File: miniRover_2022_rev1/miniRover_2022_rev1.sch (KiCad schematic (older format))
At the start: 5 parts, among them J1 XT60-M, U1 OKI

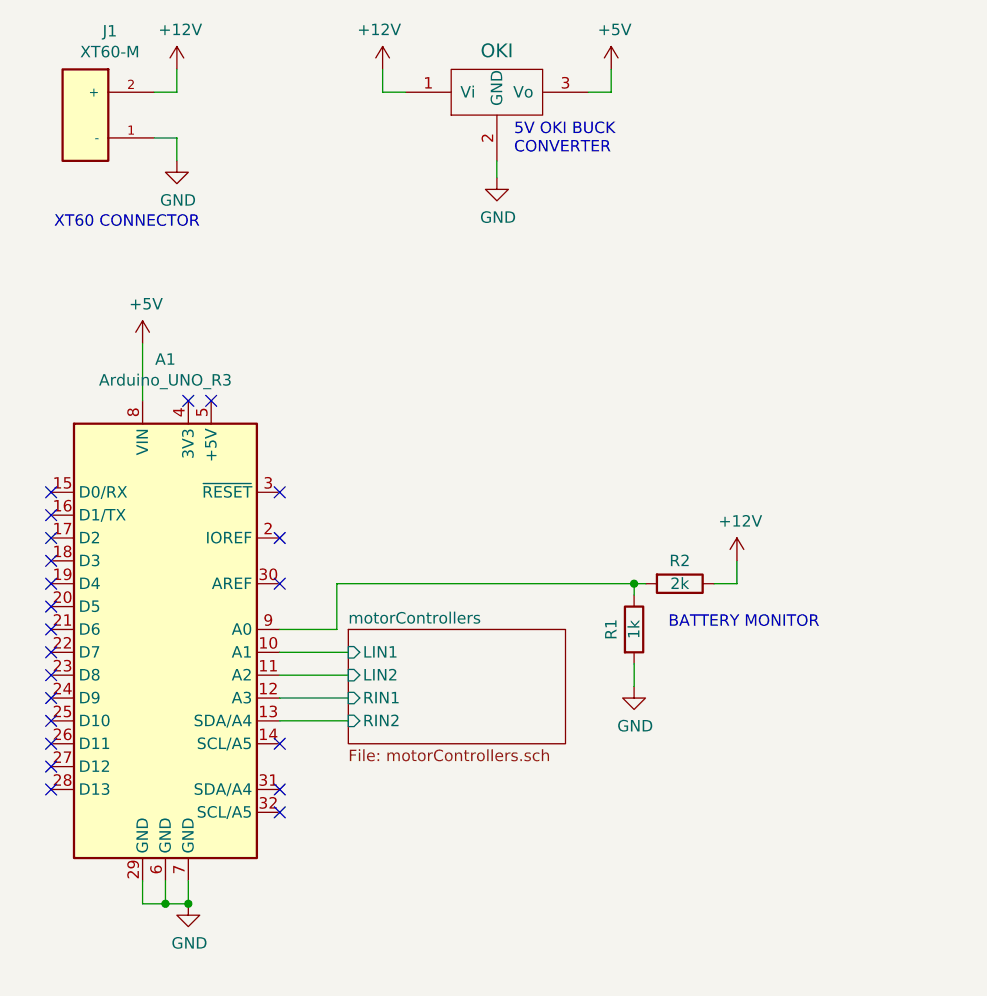
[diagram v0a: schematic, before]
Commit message: rev1 finished, will be reviewing over the following days
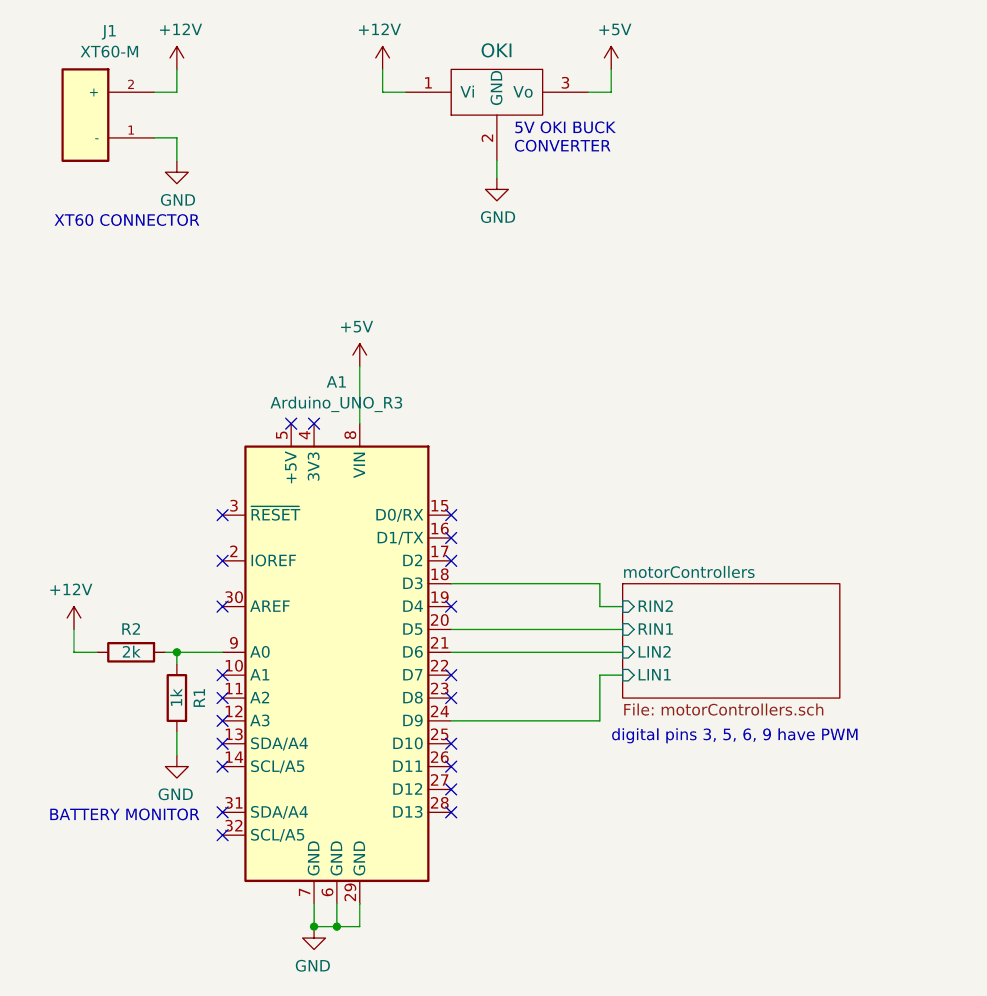
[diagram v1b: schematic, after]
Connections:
- net motorControllers/LIN1: now also A1.24 (D9); no longer A1.10 (A1)
- net motorControllers/LIN2: now also A1.21 (D6); no longer A1.11 (A2)
- net motorControllers/RIN1: now also A1.20 (D5); no longer A1.12 (A3)
- net motorControllers/RIN2: now also A1.18 (D3); no longer A1.13 (SDA/A4)
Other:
- note added: "digital pins 3, 5, 6, 9 have PWM"
- moved on the sheet: A1, R1, R2
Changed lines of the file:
@@
 Wire Wire Line
 	1100 1000 1100 1100
-$Comp
-L MCU_Module:Arduino_UNO_R3 A1
-U 1 1 60EDF96D
-P 1050 3150
-F 0 "A1" H 1050 4331 50  0000 C CNN
-F 1 "Arduino_UNO_R3" H 1050 4240 50  0000 C CNN
-F 2 "Module:Arduino_UNO_R3_WithMountingHoles" H 1050 3150 50  0001 C CIN
-F 3 "https://www.arduino.cc/en/Main/arduinoBoardUno" H 1050 3150 50  0001 C CNN
-	1    1050 3150
-	1    0    0    -1
-$EndComp
-Wire Wire Line
-	1550 3250 1850 3250
-Wire Wire Line
-	1550 3350 1850 3350
-Wire Wire Line
-	1550 3450 1850 3450
-Wire Wire Line
-	1550 3550 1850 3550
-NoConn ~ 1550 2550
-NoConn ~ 1550 2750
-NoConn ~ 1550 2950
-NoConn ~ 1550 3850
-NoConn ~ 1550 3950
+NoConn ~ 1300 2650
+NoConn ~ 1300 2850
+NoConn ~ 1300 3050
+NoConn ~ 1300 3950
+NoConn ~ 1300 4050
 $Comp
 L power:GND #PWR0106
 U 1 1 60F80F90
-P 1150 4350
-F 0 "#PWR0106" H 1150 4100 50  0001 C CNN
-F 1 "GND" H 1155 4177 50  0000 C CNN
-F 2 "" H 1150 4350 50  0001 C CNN
-F 3 "" H 1150 4350 50  0001 C CNN
-	1    1150 4350
-	1    0    0    -1
-$EndComp
-Wire Wire Line
-	950  4250 950  4350
-Wire Wire Line
-	950  4350 1050 4350
-Wire Wire Line
-	1150 4250 1150 4350
-Connection ~ 1150 4350
-Wire Wire Line
-	1050 4250 1050 4350
-Connection ~ 1050 4350
-Wire Wire Line
-	1050 4350 1150 4350
-Wire Wire Line
-	950  1900 950  2150
+P 1700 4450
+F 0 "#PWR0106" H 1700 4200 50  0001 C CNN
+F 1 "GND" H 1705 4277 50  0000 C CNN
+F 2 "" H 1700 4450 50  0001 C CNN
+F 3 "" H 1700 4450 50  0001 C CNN
+	1    1700 4450
+	-1   0    0    -1
+$EndComp
+Wire Wire Line
+	1900 4350 1900 4450
+Wire Wire Line
+	1900 4450 1800 4450
+Wire Wire Line
+	1700 4350 1700 4450
+Connection ~ 1700 4450
+Wire Wire Line
+	1800 4350 1800 4450
+Connection ~ 1800 4450
+Wire Wire Line
+	1800 4450 1700 4450
+Wire Wire Line
+	1900 2000 1900 2250
 $Comp
 L power:+5V #PWR0107
 U 1 1 60F82284
-P 950 1900
-F 0 "#PWR0107" H 950 1750 50  0001 C CNN
-F 1 "+5V" H 965 2073 50  0000 C CNN
-F 2 "" H 950 1900 50  0001 C CNN
-F 3 "" H 950 1900 50  0001 C CNN
-	1    950  1900
-	1    0    0    -1
-$EndComp
-Wire Wire Line
-	1550 3150 1800 3150
-Wire Wire Line
-	1800 3150 1800 2950
-Wire Wire Line
-	1800 2950 3100 2950
+P 1900 2000
+F 0 "#PWR0107" H 1900 1850 50  0001 C CNN
+F 1 "+5V" H 1915 2173 50  0000 C CNN
+F 2 "" H 1900 2000 50  0001 C CNN
+F 3 "" H 1900 2000 50  0001 C CNN
+	1    1900 2000
+	-1   0    0    -1
+$EndComp
 $Comp
 L Device:R R2
 U 1 1 60F82ECB
-P 3300 2950
-F 0 "R2" V 3200 2950 50  0000 C CNN
-F 1 "2k" V 3300 2950 50  0000 C CNN
-F 2 "Resistor_SMD:R_0603_1608Metric_Pad1.05x0.95mm_HandSolder" V 3230 2950 50  0001 C CNN
-F 3 "~" H 3300 2950 50  0001 C CNN
-	1    3300 2950
-	0    1    1    0
+P 900 3250
+F 0 "R2" V 800 3250 50  0000 C CNN
+F 1 "2k" V 900 3250 50  0000 C CNN
+F 2 "Resistor_SMD:R_0603_1608Metric_Pad1.05x0.95mm_HandSolder" V 830 3250 50  0001 C CNN
+F 3 "~" H 900 3250 50  0001 C CNN
+	1    900  3250
+	0    -1   1    0
 $EndComp
 $Comp
 L Device:R R1
 U 1 1 60F837E9
-P 3100 3150
-F 0 "R1" V 3000 3150 50  0000 C CNN
-F 1 "1k" V 3100 3150 50  0000 C CNN
-F 2 "Resistor_SMD:R_0603_1608Metric_Pad1.05x0.95mm_HandSolder" V 3030 3150 50  0001 C CNN
-F 3 "~" H 3100 3150 50  0001 C CNN
-	1    3100 3150
-	1    0    0    -1
-$EndComp
-Wire Wire Line
-	3100 3000 3100 2950
-Wire Wire Line
-	3150 2950 3100 2950
-Connection ~ 3100 2950
+P 1100 3450
+F 0 "R1" V 1000 3450 50  0000 C CNN
+F 1 "1k" V 1100 3450 50  0000 C CNN
+F 2 "Resistor_SMD:R_0603_1608Metric_Pad1.05x0.95mm_HandSolder" V 1030 3450 50  0001 C CNN
+F 3 "~" H 1100 3450 50  0001 C CNN
+	1    1100 3450
+	-1   0    0    -1
+$EndComp
+Wire Wire Line
+	1100 3300 1100 3250
+Wire Wire Line
+	1050 3250 1100 3250
 $Comp
 L power:GND #PWR0108
 U 1 1 60F84498
-P 3100 3400
-F 0 "#PWR0108" H 3100 3150 50  0001 C CNN
-F 1 "GND" H 3105 3227 50  0000 C CNN
-F 2 "" H 3100 3400 50  0001 C CNN
-F 3 "" H 3100 3400 50  0001 C CNN
-	1    3100 3400
-	1    0    0    -1
-$EndComp
-Wire Wire Line
-	3100 3300 3100 3400
-Wire Wire Line
-	3450 2950 3550 2950
-Wire Wire Line
-	3550 2950 3550 2850
+P 1100 3700
+F 0 "#PWR0108" H 1100 3450 50  0001 C CNN
+F 1 "GND" H 1105 3527 50  0000 C CNN
+F 2 "" H 1100 3700 50  0001 C CNN
+F 3 "" H 1100 3700 50  0001 C CNN
+	1    1100 3700
+	-1   0    0    -1
+$EndComp
+Wire Wire Line
+	1100 3600 1100 3700
+Wire Wire Line
+	750  3250 650  3250
+Wire Wire Line
+	650  3250 650  3150
 $Comp
 L power:+12V #PWR0109
 U 1 1 60F84D22
-P 3550 2850
-F 0 "#PWR0109" H 3550 2700 50  0001 C CNN
-F 1 "+12V" H 3565 3023 50  0000 C CNN
-F 2 "" H 3550 2850 50  0001 C CNN
-F 3 "" H 3550 2850 50  0001 C CNN
-	1    3550 2850
-	1    0    0    -1
-$EndComp
-NoConn ~ 550  3850
-NoConn ~ 550  3750
-NoConn ~ 550  3650
-NoConn ~ 550  3550
-NoConn ~ 550  3450
-NoConn ~ 550  3350
-NoConn ~ 550  3250
-NoConn ~ 550  3150
-NoConn ~ 550  3050
-NoConn ~ 550  2950
-NoConn ~ 550  2850
-NoConn ~ 550  2750
-NoConn ~ 550  2650
-NoConn ~ 550  2550
-NoConn ~ 1550 3650
+P 650 3150
+F 0 "#PWR0109" H 650 3000 50  0001 C CNN
+F 1 "+12V" H 665 3323 50  0000 C CNN
+F 2 "" H 650 3150 50  0001 C CNN
+F 3 "" H 650 3150 50  0001 C CNN
+	1    650  3150
+	-1   0    0    -1
+$EndComp
+NoConn ~ 2300 3950
+NoConn ~ 2300 3850
+NoConn ~ 2300 3750
+NoConn ~ 2300 3650
+NoConn ~ 2300 3450
+NoConn ~ 2300 3350
+NoConn ~ 2300 3050
+NoConn ~ 2300 2850
+NoConn ~ 2300 2750
+NoConn ~ 2300 2650
+NoConn ~ 1300 3750
 Text Notes 1200 1400 2    50   ~ 0
 XT60 CONNECTOR\n
@@
 Text Notes 2575 1075 0    50   ~ 0
 5V OKI BUCK\nCONVERTER
-Text Notes 3250 3150 0    50   ~ 0
+Text Notes 1200 4000 2    50   ~ 0
 BATTERY MONITOR
 $Sheet
-S 1850 3150 950  500
+S 3050 2950 950  500
 U 60F3E927
 F0 "motorControllers" 50
 F1 "motorControllers.sch" 50
-F2 "LIN1" I L 1850 3250 50
-F3 "LIN2" I L 1850 3350 50
-F4 "RIN1" I L 1850 3450 50
-F5 "RIN2" I L 1850 3550 50
+F2 "LIN1" I L 3050 3350 50
+F3 "LIN2" I L 3050 3250 50
+F4 "RIN1" I L 3050 3150 50
+F5 "RIN2" I L 3050 3050 50
 $EndSheet
-NoConn ~ 1150 2150
-NoConn ~ 1250 2150
+NoConn ~ 1700 2250
+NoConn ~ 1600 2250
+$Comp
+L MCU_Module:Arduino_UNO_R3 A1
+U 1 1 60EDF96D
+P 1800 3250
+F 0 "A1" H 1800 4431 50  0000 C CNN
+F 1 "Arduino_UNO_R3" H 1800 4340 50  0000 C CNN
+F 2 "Module:Arduino_UNO_R3_WithMountingHoles" H 1800 3250 50  0001 C CIN
+F 3 "https://www.arduino.cc/en/Main/arduinoBoardUno" H 1800 3250 50  0001 C CNN
+	1    1800 3250
+	-1   0    0    -1
+$EndComp
+Wire Wire Line
+	1300 3250 1100 3250
+Connection ~ 1100 3250
+NoConn ~ 1300 3350
+NoConn ~ 1300 3450
+NoConn ~ 1300 3550
+NoConn ~ 1300 3650
+Text Notes 3000 3650 0    50   ~ 0
+digital pins 3, 5, 6, 9 have PWM
+Wire Wire Line
+	3050 3250 2300 3250
+Wire Wire Line
+	2300 3150 3050 3150
+Wire Wire Line
+	3050 3050 2950 3050
+Wire Wire Line
+	2950 3050 2950 2950
+Wire Wire Line
+	2950 2950 2300 2950
+Wire Wire Line
+	2300 3550 2950 3550
+Wire Wire Line
+	2950 3550 2950 3350
+Wire Wire Line
+	2950 3350 3050 3350
 $EndSCHEMATC
